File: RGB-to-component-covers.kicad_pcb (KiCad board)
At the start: 2 copper layers, 58.9 x 150.6 mm, 22 parts

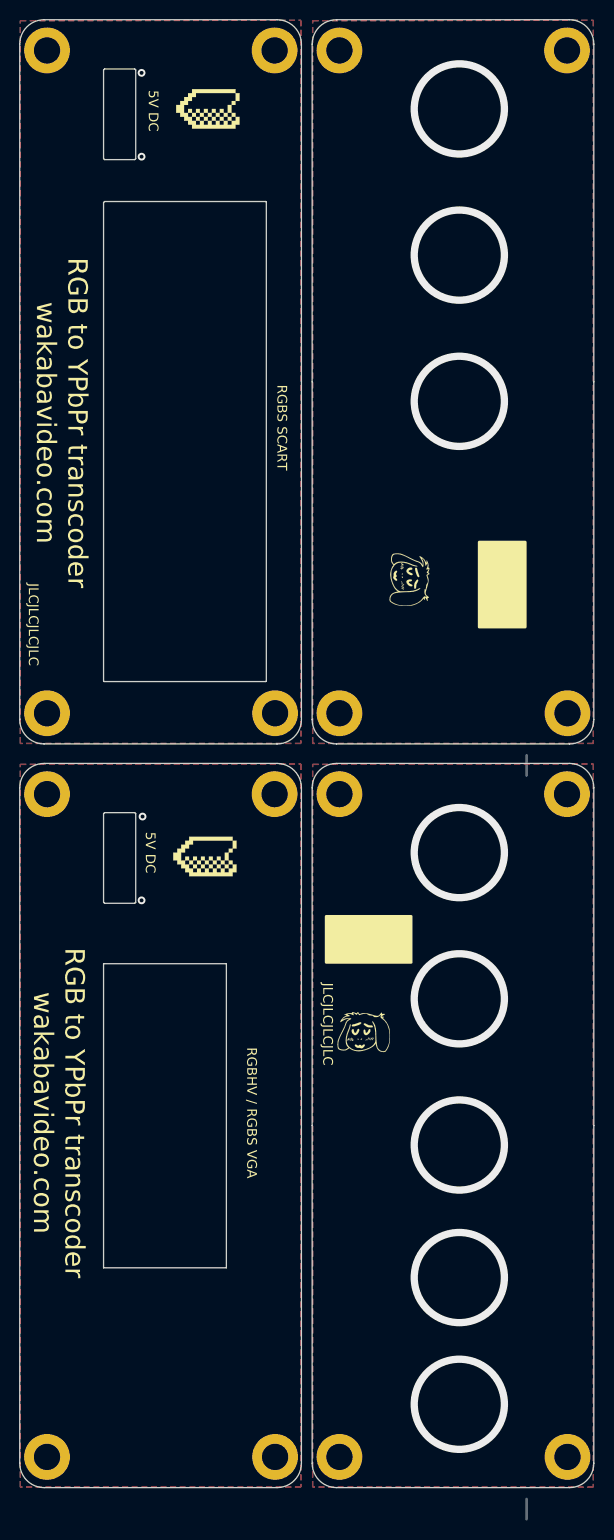
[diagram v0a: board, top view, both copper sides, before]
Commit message: covers updated
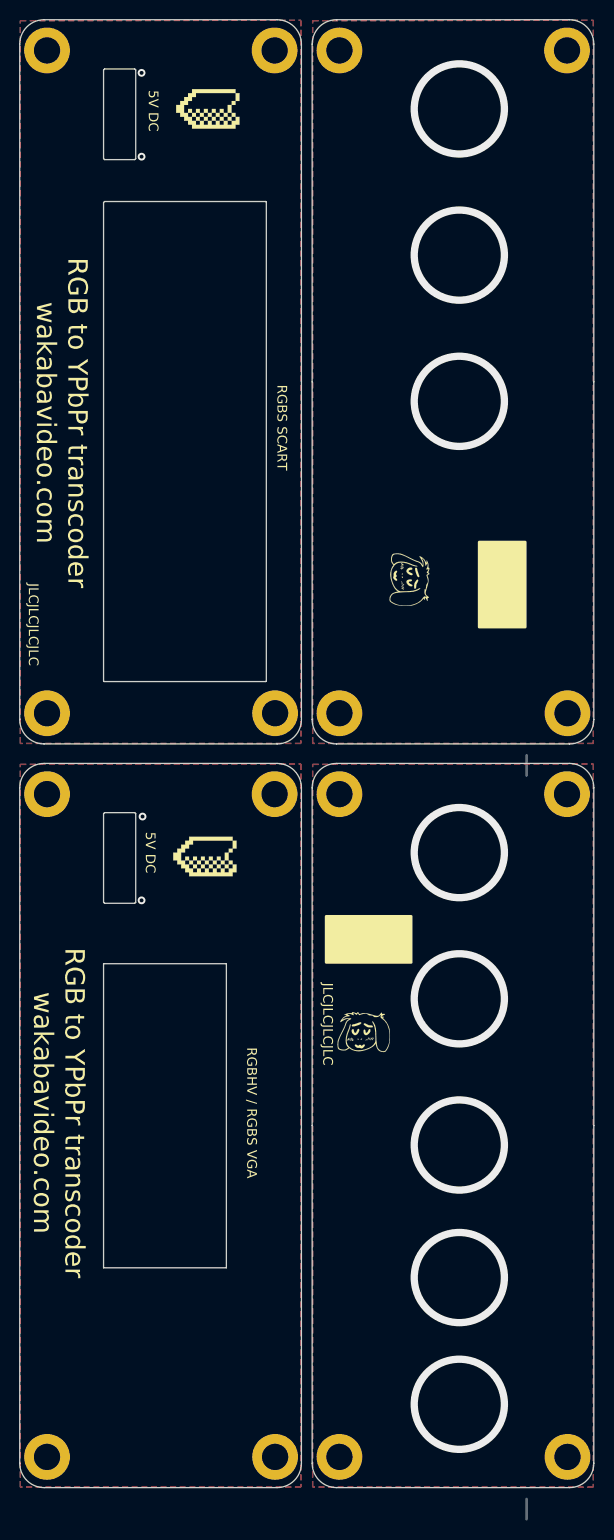
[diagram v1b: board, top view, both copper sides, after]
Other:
- net class Default removed
